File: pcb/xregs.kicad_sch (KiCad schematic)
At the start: 13 parts

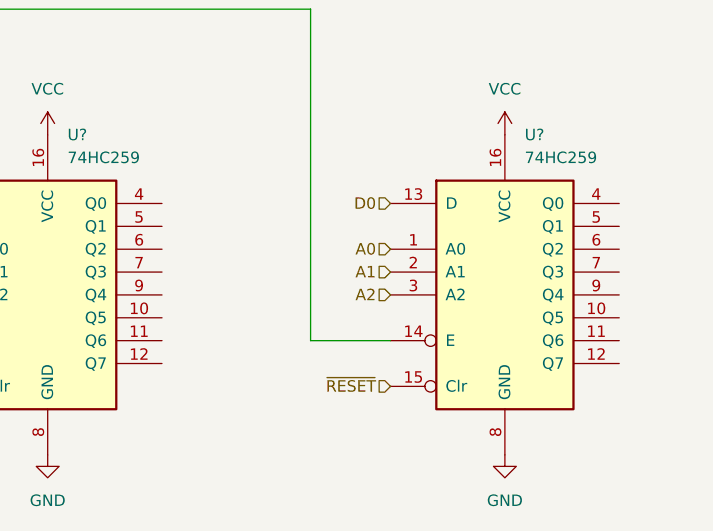
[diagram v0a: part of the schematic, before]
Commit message: WIP schematic
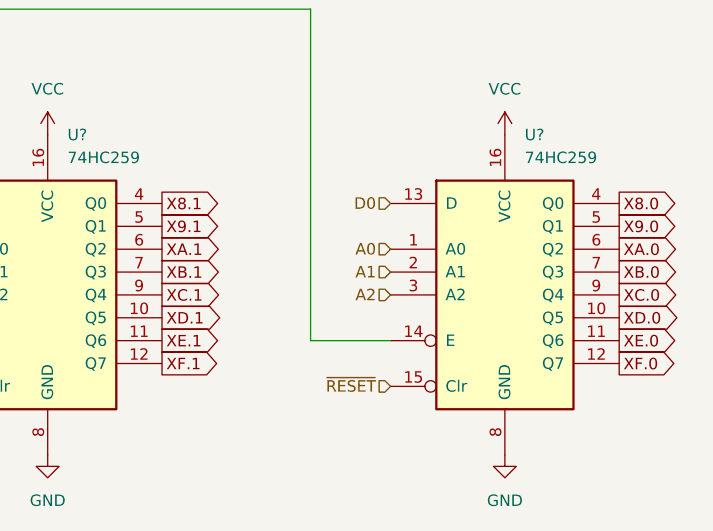
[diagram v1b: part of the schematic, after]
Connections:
- net XD.0: now reaches U?.10 (Q5)
- net XE.0: now reaches U?.11 (Q6)
- net XF.0: now reaches U?.12 (Q7)
- net X8.0: now reaches U?.4 (Q0)
- net X9.0: now reaches U?.5 (Q1)
- net XA.0: now reaches U?.6 (Q2)
- net XB.0: now reaches U?.7 (Q3)
- net XC.0: now reaches U?.9 (Q4)
- net XD.1: now reaches U?.10 (Q5)
- net XE.1: now reaches U?.11 (Q6)
- net XF.1: now reaches U?.12 (Q7)
- net X8.1: now reaches U?.4 (Q0)
- net X9.1: now reaches U?.5 (Q1)
- net XA.1: now reaches U?.6 (Q2)
- net XB.1: now reaches U?.7 (Q3)
- net XC.1: now reaches U?.9 (Q4)
